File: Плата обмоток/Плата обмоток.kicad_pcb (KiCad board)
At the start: 2 copper layers, 58 x 58 mm, 7 parts, among them J1 A_OUT, J2 B_OUT, J3 C_OUT, J4 Conn_01x02, J5 Conn_02x02_Odd_Even, J6 Conn_01x02, J7 Conn_01x02

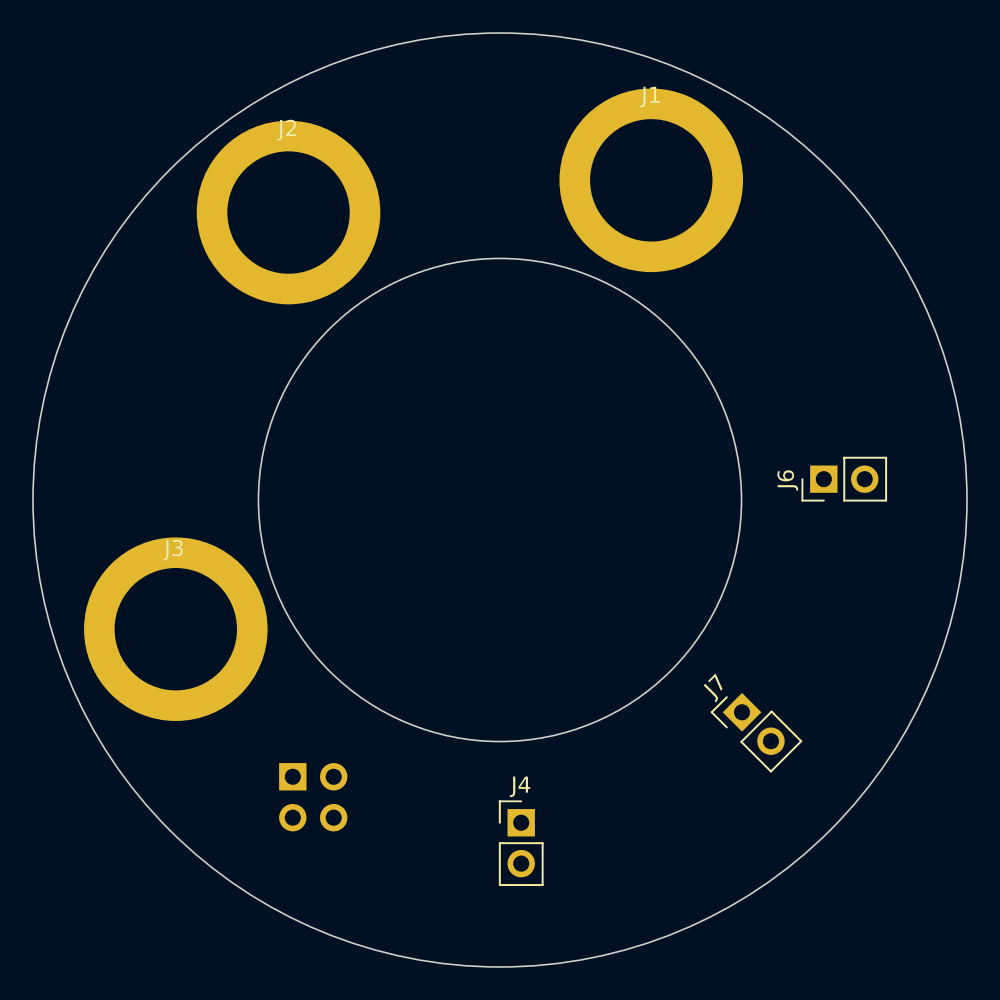
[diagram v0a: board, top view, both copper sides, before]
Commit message: Добавил ножевые разъёмы
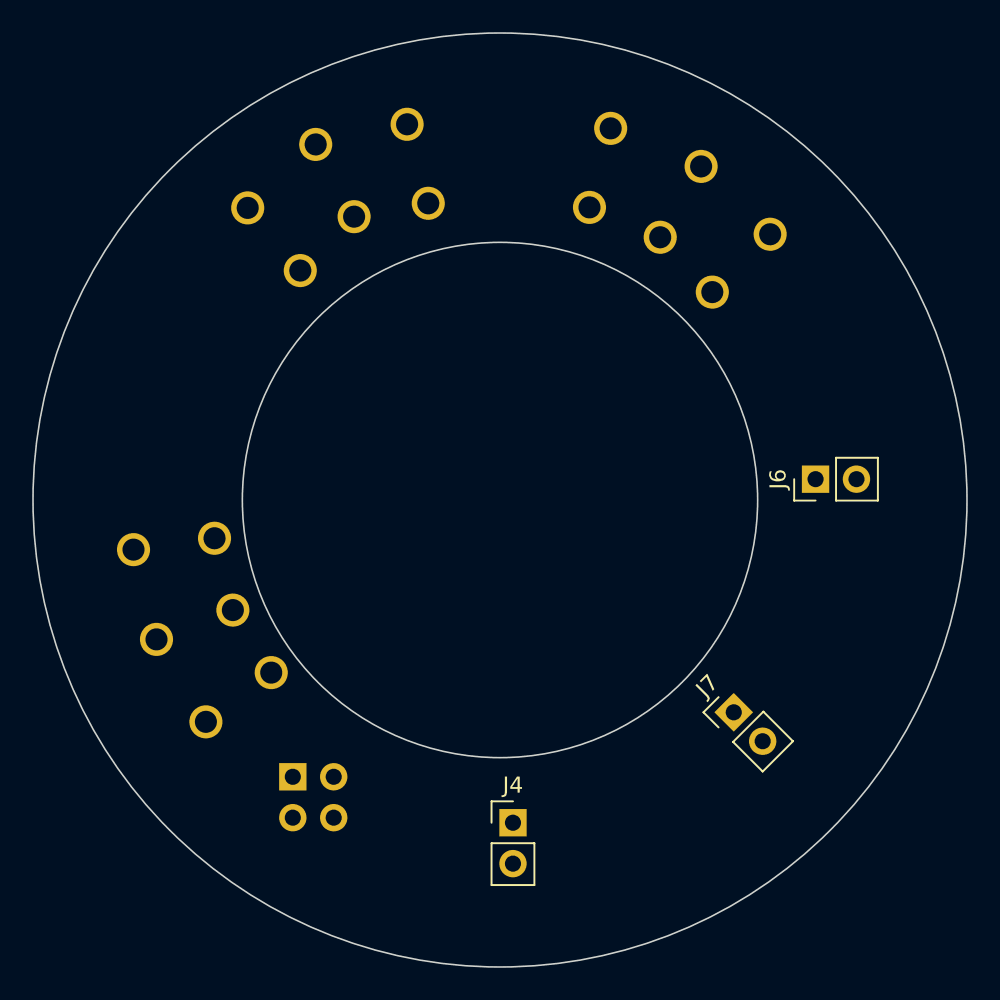
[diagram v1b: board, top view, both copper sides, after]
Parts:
- added J10: 4900, Connector_My:3551, B.Cu at (70.9, 81.8)
- added J11: 4900, Connector_My:3551, B.Cu at (60.5, 99.1)
- added J12: 4900, Connector_My:3551, B.Cu at (61.9, 104.7)
- added J13: 4900, Connector_My:3551, B.Cu at (65.0, 109.8)
- added J8: 4900, Connector_My:3551, B.Cu at (78.8, 77.6)
- added J9: 4900, Connector_My:3551, B.Cu at (74.2, 78.4)
- J1: value A_OUT -> 4900; footprint Connector_My:Power_Wire -> Connector_My:3551; moved to B.Cu
- J2: value B_OUT -> 4900; footprint Connector_My:Power_Wire -> Connector_My:3551; moved to B.Cu
- J3: value C_OUT -> 4900; footprint Connector_My:Power_Wire -> Connector_My:3551; moved to B.Cu
- moved J3 39.3 mm to (96.5, 83.1), turned to 45 degrees
- moved J2 23.1 mm to (93.2, 79.7), turned to 60 degrees
- moved J1 4.19 mm to (88.8, 77.9), turned to 75 degrees
- moved J4 0.51 mm to (84.1, 116.1)
- moved J6 0.51 mm to (102.9, 94.7)
- moved J7 0.51 mm to (97.8, 109.2)
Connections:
- J2 pad 1: B_OUT -> A_OUT
- J3 pad 1: C_OUT -> A_OUT
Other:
- outline, holes or cut-outs redrawn
